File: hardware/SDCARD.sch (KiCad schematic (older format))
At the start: 7 parts, among them J6 TF_HEADER, U3 CD74HC4050, U4 TF_CARD_SOCKET,SELF_EJECT

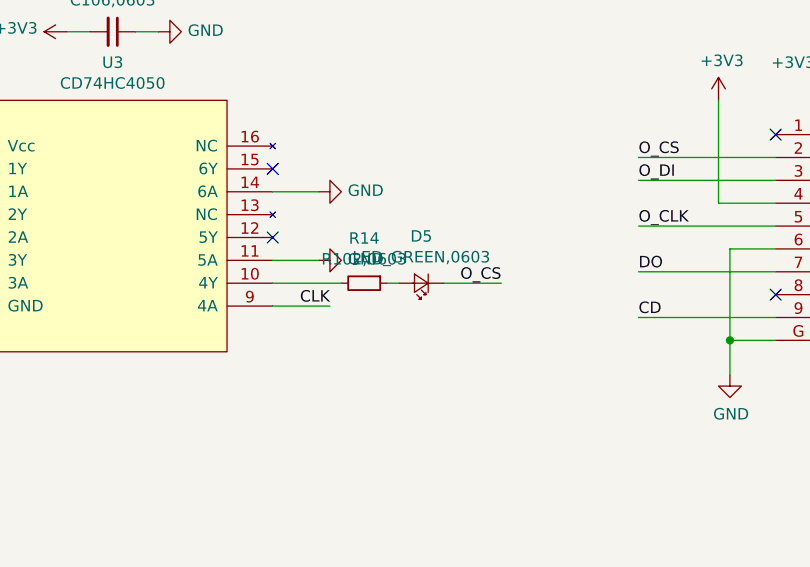
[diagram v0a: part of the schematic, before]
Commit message: update,
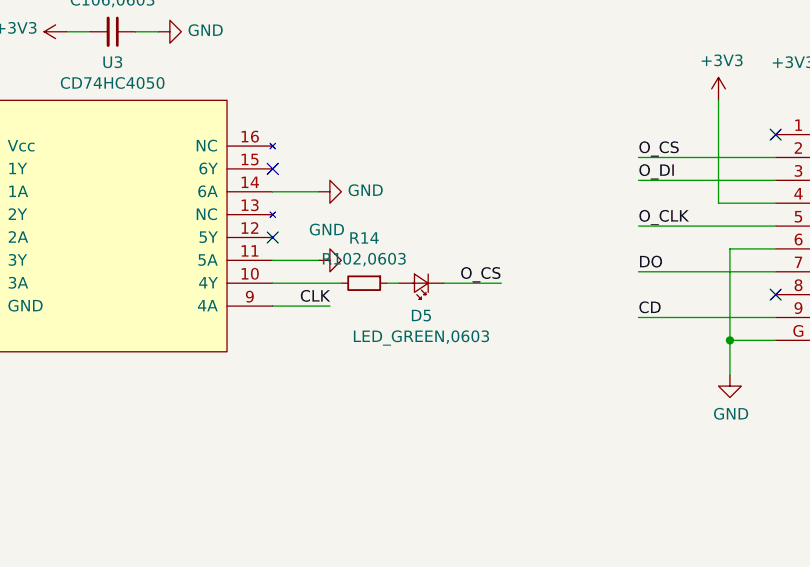
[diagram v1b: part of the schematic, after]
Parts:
- U3: footprint (none) -> footprint-lib:74HCT4050_SOP16
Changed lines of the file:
@@
 U 1 1 5CFEA629
 P 4200 2550
-F 0 "D5" H 4200 2345 50  0000 C CNN
-F 1 "LED_GREEN,0603" H 4200 2436 50  0000 C CNN
+F 0 "D5" H 4200 2693 50  0000 C CNN
+F 1 "LED_GREEN,0603" H 4200 2784 50  0000 C CNN
 F 2 "footprint-lib:LED_0603_1608Metric" V 4200 2550 50  0001 C CNN
 F 3 "" V 4200 2550 50  0001 C CNN
@@
 P 3750 2450
 F 0 "#PWR041" H 3750 2200 50  0001 C CNN
-F 1 "GND" V 3755 2322 50  0000 R CNN
+F 1 "GND" V 3883 2413 50  0000 C CNN
 F 2 "" H 3750 2450 50  0001 C CNN
 F 3 "" H 3750 2450 50  0001 C CNN
@@
 Text Label 1700 2350 0    50   ~ 0
 DI
-$Comp
-L taobao-components:CD74HC4050 U3
-U 1 1 5CFD5C32
-P 2850 2300
-F 0 "U3" H 2850 3015 50  0000 C CNN
-F 1 "CD74HC4050" H 2850 2924 50  0000 C CNN
-F 2 "" H 2850 2300 50  0001 C CNN
-F 3 "" H 2850 2300 50  0001 C CNN
-	1    2850 2300
-	1    0    0    -1
-$EndComp
 Wire Wire Line
 	1600 1000 1150 1000
@@
 EndData
 $EndBitmap
+$Comp
+L taobao-components:CD74HC4050 U3
+U 1 1 5CF97526
+P 2850 2300
+F 0 "U3" H 2850 3015 50  0000 C CNN
+F 1 "CD74HC4050" H 2850 2924 50  0000 C CNN
+F 2 "footprint-lib:74HCT4050_SOP16" H 2850 1500 50  0001 C CNN
+F 3 "" H 2850 2300 50  0001 C CNN
+	1    2850 2300
+	1    0    0    -1
+$EndComp
 $EndSCHEMATC
